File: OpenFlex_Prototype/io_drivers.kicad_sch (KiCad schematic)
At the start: 29 parts, among them Q1 IRF740, Q2 IRF740, Q3 IRF740, Q4 IRF740, U2 LM324, U3 TC4424, U4 TC4424

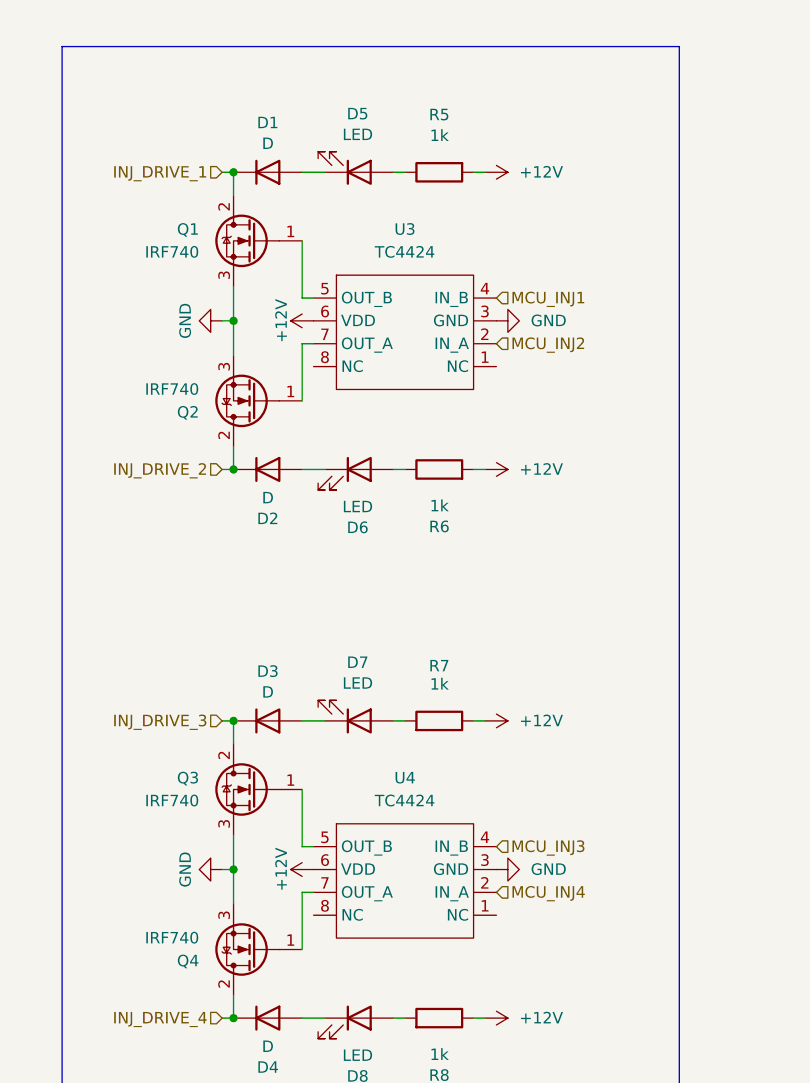
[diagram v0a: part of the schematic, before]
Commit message: Updated Sourcing for prototype
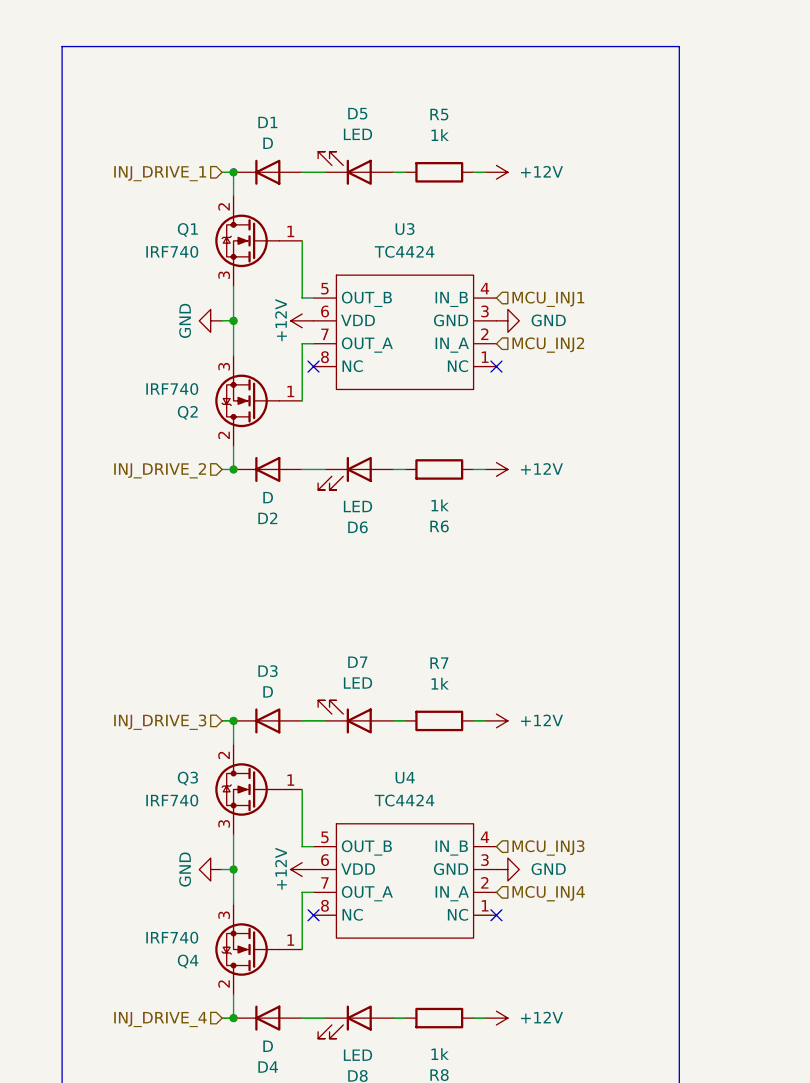
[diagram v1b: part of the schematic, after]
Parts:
- C1: Digikey Part Number 445-180563-1-ND -> (none); URL https://www.digikey.com.au/product-detail/en/tdk-corporatio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 -> https://www.mouser.fr/ProductDetail/TDK/FA18X8R1E104KNU06?q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
- C2, C3: Digikey Part Number Digikey Part Number -> (none); URL https://www.digikey.com.au/product-detail/en/tdk-corporatio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 -> https://www.mouser.fr/ProductDetail/TDK/FA18X8R1E224KRU06?q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
- D7: Digikey Part Number 732-5005-ND -> (none)
- R1, R2, R3, R4: Manufacturer_Name (none) -> YAGEO; Manufacturer_Part_Number (none) -> MFR-25FBF52-10K; Mouser_Part_Number (none) -> 603-MFR-25FBF52-10K; URL (none) -> https://www.mouser.fr/ProductDetail/YAGEO/MFR-25FBF52-10K?q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
- R10: Digikey Part Number P470CCT-ND -> (none); Manufacturer_Name Panasonic -> YAGEO; Manufacturer_Part_Number ERJ-6ENF4700V -> MFR-25FTE52-470R; Mouser_Part_Number (none) -> 603-MFR-25FTE52-470R; URL https://www.digikey.com/product-detail/en/panasonic-electro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 -> https://www.mouser.fr/ProductDetail/YAGEO/MFR-25FTE52-470R?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
- R11: Digikey Part Number 311-2.40KCRCT-ND -> (none); Manufacturer_Part_Number RC0805FR-072K4L -> MFR-25FBF52-2K4; Mouser_Part_Number (none) -> 603-MFR-25FBF52-2K4; URL https://www.digikey.com/product-detail/en/yageo/RC0805FR-07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 -> https://www.mouser.fr/ProductDetail/YAGEO/MFR-25FBF52-2K4?q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
- R5, R6, R7, R8: Digikey Part Number 311-1.00KCRCT-ND -> (none); Manufacturer_Name Yageo -> YAGEO; Manufacturer_Part_Number RC0805FR-071KL -> MFR-25FBF52-1K; Mouser_Part_Number (none) -> 603-MFR-25FBF52-1K; URL https://www.digikey.com/product-detail/en/yageo/RC0805FR-07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 -> https://www.mouser.fr/ProductDetail/YAGEO/MFR-25FBF52-1K?qs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
- R9: Digikey Part Number YAG1854CT-ND -> (none); Manufacturer_Part_Number RT0805BRD072K49L -> MFR-25FBF52-2K49; Mouser_Part_Number (none) -> 603-MFR-25FBF52-2K49; URL https://www.digikey.com/product-detail/en/yageo/RT0805BRD07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 -> https://www.mouser.fr/ProductDetail/YAGEO/MFR-25FBF52-2K49?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
- U2: Manufacturer Texas Instrument -> (none); Manufacturer part number LM324KAN -> (none); Manufacturer_Name (none) -> Texas Instrument; Manufacturer_Part_Number (none) -> LM324KAN; Mouser link https://www.mouser.fr/ProductDetail/Texas-Instruments/LM324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 -> (none); Mouser part Number 595-LM324KAN -> (none); Mouser_Part_Number (none) -> 595-LM324KAN; URL (none) -> https://www.mouser.fr/ProductDetail/Texas-Instruments/LM324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
- U3, U4: Manufacturer Microchip Technology -> (none); Manufacturer part number TC4424AVPA -> (none); Manufacturer_Name (none) -> Microchip Technology; Manufacturer_Part_Number (none) -> TC4424AVPA; Mouser link https://www.mouser.fr/ProductDetail/Microchip-Technology/TC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 -> (none); Mouser part number 579-TC4424AVPA -> (none); Mouser_Part_Number (none) -> 579-TC4424AVPA; URL (none) -> https://www.mouser.fr/ProductDetail/Microchip-Technology/TC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
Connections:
- net +12V: now also R5.1, R6.1; no longer R5.2, R6.2
- net at D5.2 (A): now also R5.2; no longer R5.1
- net at D6.2 (A): now also R6.2; no longer R6.1
- no-connect marks 0 -> 4
